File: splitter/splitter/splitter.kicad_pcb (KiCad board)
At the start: 2 copper layers, 50.8 x 63 mm, 33 parts, among them J1 JACKIN, J2 JACKSEND, J3 JACKRECV, J4 JACKOUT, J5 Jack-DC, J6 CONN_SEND_DRY, J7 RING_SEND, J8 CONN_RECV_DRY, J9 RING_RECV, SW1 SW_MODE, SW2 SW_BYPASS, U1 TL074, U2 TLE2426xLP

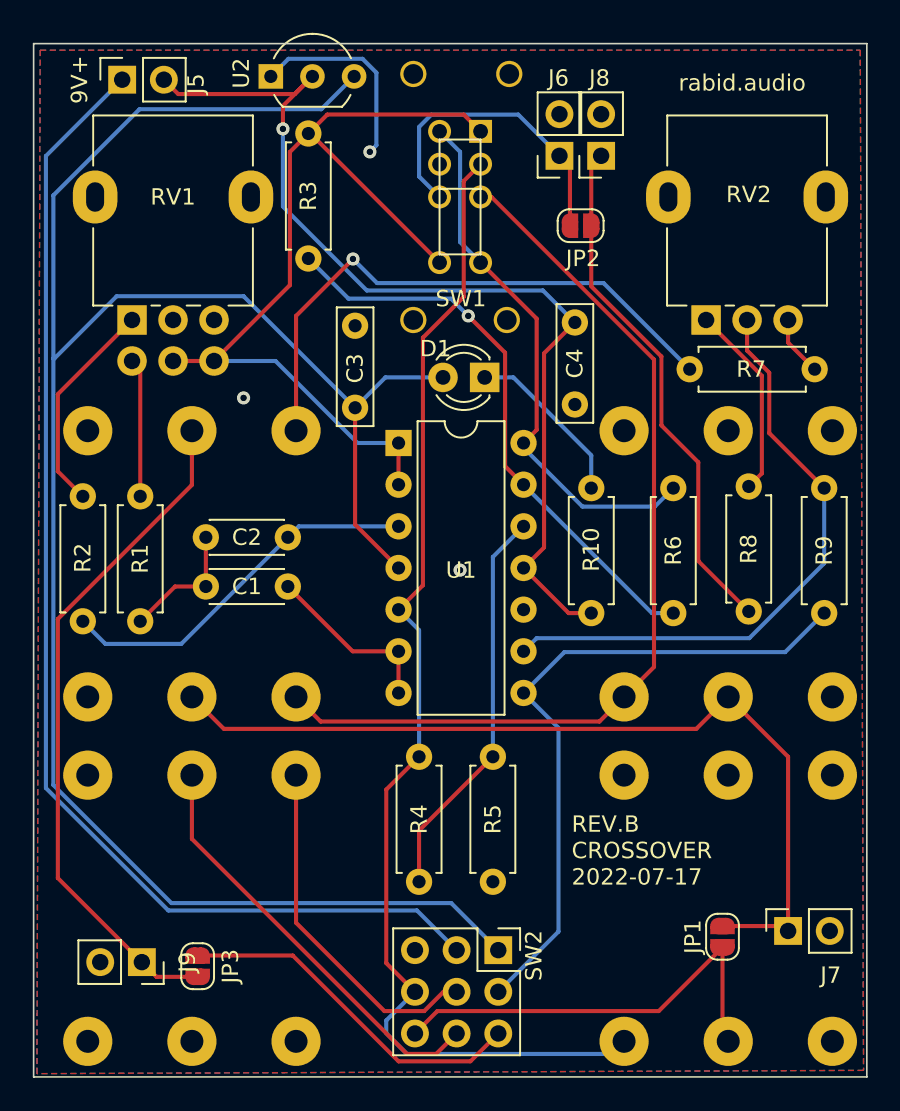
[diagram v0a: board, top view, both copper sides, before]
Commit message: cleanup
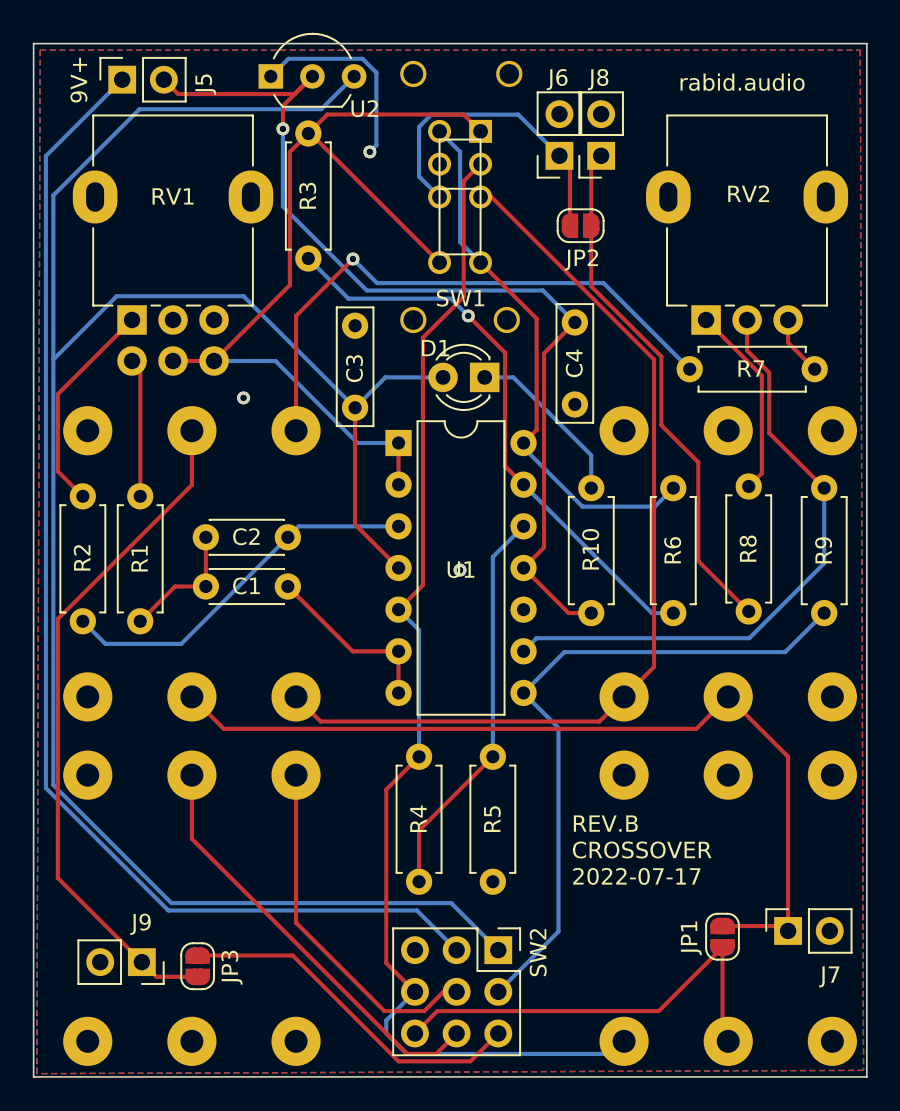
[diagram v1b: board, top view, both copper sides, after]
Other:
- board text added: "21mm between jacks 61.5mm internal width, 2mm walls"
- board text removed: "21mm between jacks 61.5mm internal width, 2mm walls, 60mm board width jack sleve 4mm. thus needs 2-(1.5/2) = 1.25mm inset"
